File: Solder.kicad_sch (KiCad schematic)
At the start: 5 parts

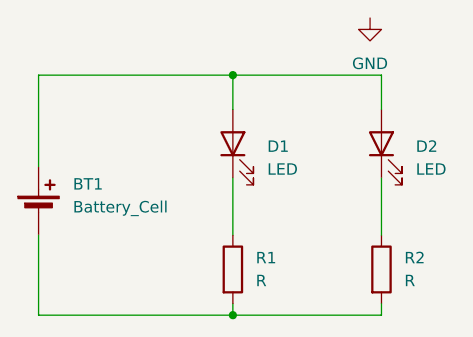
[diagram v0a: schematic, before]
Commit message: Finished? :D
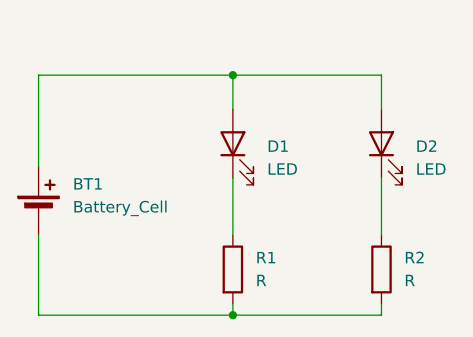
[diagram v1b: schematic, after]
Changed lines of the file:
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@@
-	)
-	(symbol
-		(lib_id "power:GND")
-		(at 142.24 57.15 0)
-		(unit 1)
-		(exclude_from_sim no)
-		(in_bom yes)
-		(on_board yes)
-		(dnp no)
-		(fields_autoplaced yes)
-		(property "Reference" "#PWR01"
-			(at 142.24 63.5 0)
-			(effects
-				(font
-					(size 1.27 1.27)
-				)
-				(hide yes)
-			)
-		)
-		(property "Value" "GND"
-			(at 142.24 62.23 0)
-			(effects
-				(font
-					(size 1.27 1.27)
-				)
-			)
-		)
-		(property "Footprint" ""
-			(at 142.24 57.15 0)
-			(effects
-				(font
-					(size 1.27 1.27)
-				)
-				(hide yes)
-			)
-		)
-		(property "Datasheet" ""
-			(at 142.24 57.15 0)
-			(effects
-				(font
-					(size 1.27 1.27)
-				)
-				(hide yes)
-			)
-		)
-		(property "Description" "Power symbol creates a global label with name \"GND\" , ground"
-			(at 142.24 57.15 0)
-			(effects
-				(font
-					(size 1.27 1.27)
-				)
-				(hide yes)
-			)
-		)
-		(pin "1"
-		)
-		(instances
-			(project ""
-				(path "/8b732828-8244-451f-9bdb-50d32063189d"
-					(reference "#PWR01")
-					(unit 1)
-				)
-			)
-		)
 	)
 	(symbol
